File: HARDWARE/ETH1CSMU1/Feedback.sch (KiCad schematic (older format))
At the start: 91 parts, among them K301 CRR05-1A, K302 CRR05-1A, K303 CRR05-1A, K304 CRR05-1A, K305 CRR05-1A, K306 CRR05-1A, Q301 MMBT6429, Q302 MMBT6429, Q303 MMBT6429, Q304 MMBT6429, Q305 Q_NJFET_DGS, Q306 Q_NJFET_DGS, Q307 Q_NJFET_DGS, U301 AD746, U302 AQY221, U303 AQY221, U304 AQY221, U305 AQY221, U306 AQY221, U307 AQY221, U308 ADA4530-1, U309 AD746, U310 AD744, U311 AQY221, U312 AQY221, U313 AD744, U314 AQY221, U315 AD744, U316 REF102CU, U317 OPA277

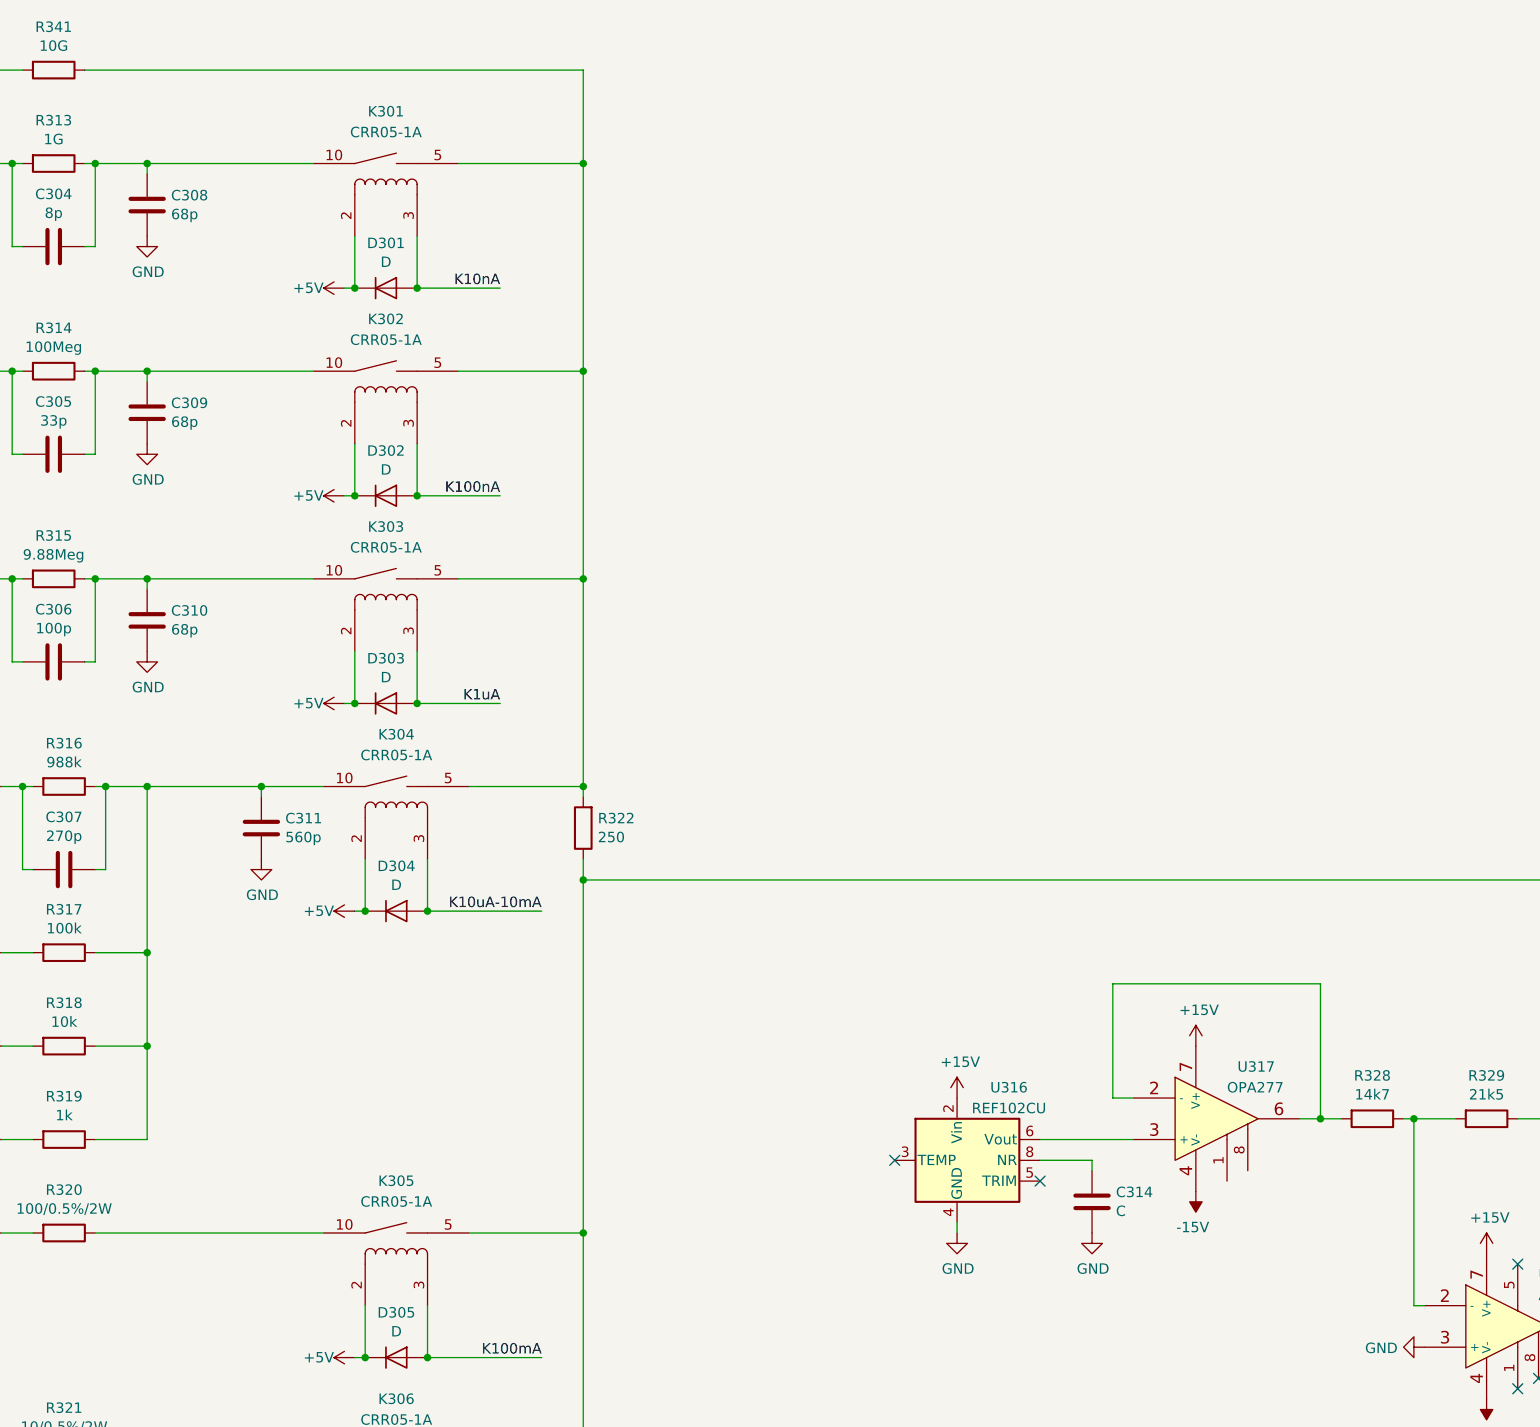
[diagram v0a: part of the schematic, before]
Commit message: Commit
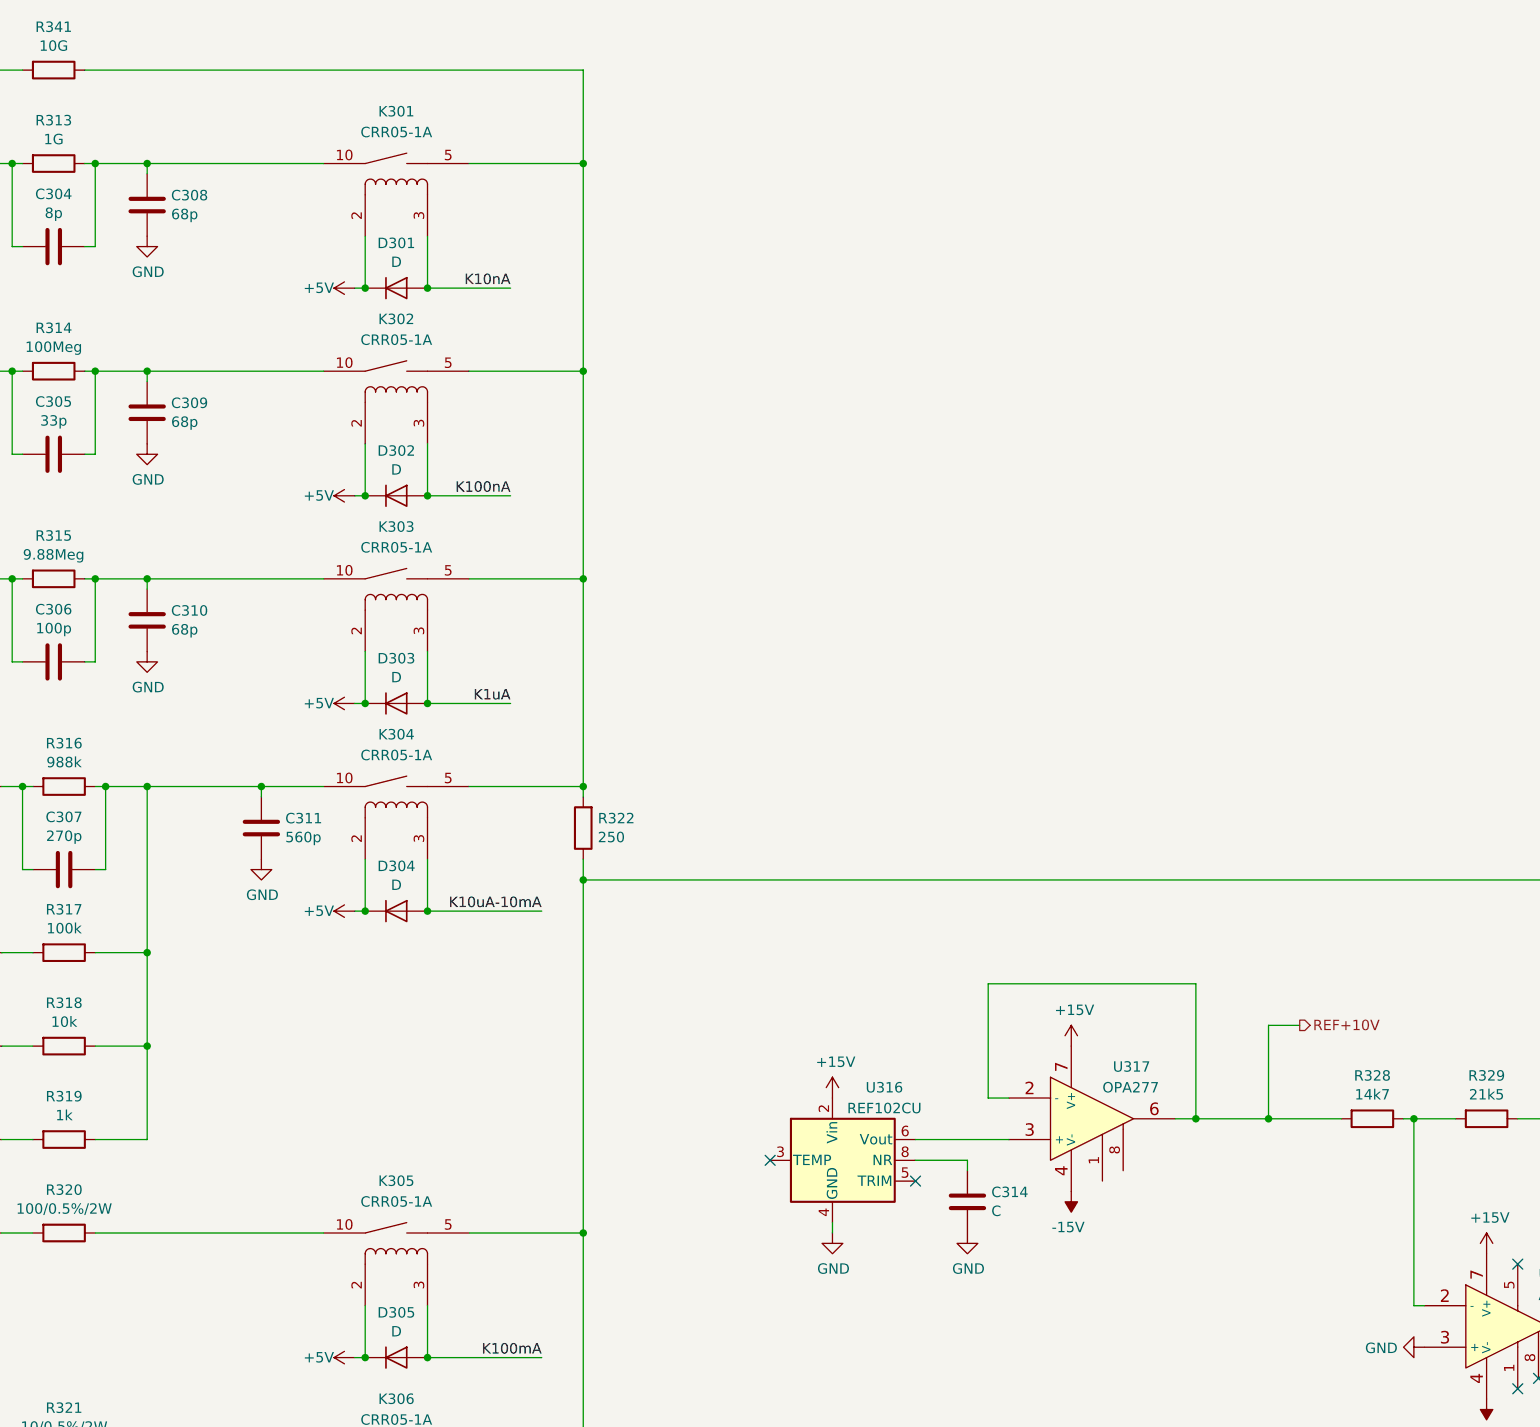
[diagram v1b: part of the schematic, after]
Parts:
- R310, R312, R318: footprint (none) -> SMD:R_0603_Symbol1
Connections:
- net REF+10V: now reaches R328.2, U317.2 (-), U317.6
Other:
- moved on the sheet: C314, D301, D302, D303, K301, K302, K303, U316, U317

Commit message: Footprints
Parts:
- C301, C302: footprint (none) -> SMD:C_0603_Symbol5
- C303, C304, C305, C308, C309, C310, C312: footprint (none) -> Capacitors_SMD:C_0603
- R305, R307, R309, R311, R317, R324: footprint (none) -> SMD:R_0603_Symbol3
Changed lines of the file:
@@
 F 0 "C305" V 5348 3300 50  0000 C CNN
 F 1 "33p" V 5439 3300 50  0000 C CNN
-F 2 "" H 5638 3150 50  0001 C CNN
+F 2 "Capacitors_SMD:C_0603" H 5638 3150 50  0001 C CNN
 F 3 "~" H 5600 3300 50  0001 C CNN
 	1    5600 3300
@@
 F 0 "R311" V 4143 8300 50  0000 C CNN
 F 1 "100k" V 4234 8300 50  0000 C CNN
-F 2 "" V 4280 8300 50  0001 C CNN
+F 2 "SMD:R_0603_Symbol3" V 4280 8300 50  0001 C CNN
 F 3 "~" H 4350 8300 50  0001 C CNN
 	1    4350 8300
@@
 F 0 "C302" V 4098 8650 50  0000 C CNN
 F 1 "15p" V 4189 8650 50  0000 C CNN
-F 2 "" H 4388 8500 50  0001 C CNN
+F 2 "SMD:C_0603_Symbol5" H 4388 8500 50  0001 C CNN
 F 3 "~" H 4350 8650 50  0001 C CNN
 	1    4350 8650
@@
 F 0 "R309" V 3743 8300 50  0000 C CNN
 F 1 "100k" V 3834 8300 50  0000 C CNN
-F 2 "" V 3880 8300 50  0001 C CNN
+F 2 "SMD:R_0603_Symbol3" V 3880 8300 50  0001 C CNN
 F 3 "~" H 3950 8300 50  0001 C CNN
 	1    3950 8300
@@
 F 0 "C301" V 3698 8650 50  0000 C CNN
 F 1 "15p" V 3789 8650 50  0000 C CNN
-F 2 "" H 3988 8500 50  0001 C CNN
+F 2 "SMD:C_0603_Symbol5" H 3988 8500 50  0001 C CNN
 F 3 "~" H 3950 8650 50  0001 C CNN
 	1    3950 8650
@@
 F 0 "C303" H 4665 9546 50  0000 L CNN
 F 1 "39p" H 4665 9455 50  0000 L CNN
-F 2 "" H 4588 9350 50  0001 C CNN
+F 2 "Capacitors_SMD:C_0603" H 4588 9350 50  0001 C CNN
 F 3 "~" H 4550 9500 50  0001 C CNN
 	1    4550 9500
@@
 F 0 "R307" V 2843 9100 50  0000 C CNN
 F 1 "100k" V 2934 9100 50  0000 C CNN
-F 2 "" V 2980 9100 50  0001 C CNN
+F 2 "SMD:R_0603_Symbol3" V 2980 9100 50  0001 C CNN
 F 3 "~" H 3050 9100 50  0001 C CNN
 	1    3050 9100
@@
 F 0 "R305" V 2193 8800 50  0000 C CNN
 F 1 "100k" V 2284 8800 50  0000 C CNN
-F 2 "" V 2330 8800 50  0001 C CNN
+F 2 "SMD:R_0603_Symbol3" V 2330 8800 50  0001 C CNN
 F 3 "~" H 2400 8800 50  0001 C CNN
 	1    2400 8800
@@
 F 0 "C309" H 6165 3146 50  0000 L CNN
 F 1 "68p" H 6165 3055 50  0000 L CNN
-F 2 "" H 6088 2950 50  0001 C CNN
+F 2 "Capacitors_SMD:C_0603" H 6088 2950 50  0001 C CNN
 F 3 "~" H 6050 3100 50  0001 C CNN
 	1    6050 3100
@@
 F 0 "C310" H 6165 4146 50  0000 L CNN
 F 1 "68p" H 6165 4055 50  0000 L CNN
-F 2 "" H 6088 3950 50  0001 C CNN
+F 2 "Capacitors_SMD:C_0603" H 6088 3950 50  0001 C CNN
 F 3 "~" H 6050 4100 50  0001 C CNN
 	1    6050 4100
@@
 F 0 "R317" V 5443 5700 50  0000 C CNN
 F 1 "100k" V 5534 5700 50  0000 C CNN
-F 2 "" V 5580 5700 50  0001 C CNN
+F 2 "SMD:R_0603_Symbol3" V 5580 5700 50  0001 C CNN
 F 3 "~" H 5650 5700 50  0001 C CNN
 	1    5650 5700
@@
 F 0 "C304" V 5348 2300 50  0000 C CNN
 F 1 "8p" V 5439 2300 50  0000 C CNN
-F 2 "" H 5638 2150 50  0001 C CNN
+F 2 "Capacitors_SMD:C_0603" H 5638 2150 50  0001 C CNN
 F 3 "~" H 5600 2300 50  0001 C CNN
 	1    5600 2300
@@
 F 0 "C308" H 6165 2146 50  0000 L CNN
 F 1 "68p" H 6165 2055 50  0000 L CNN
-F 2 "" H 6088 1950 50  0001 C CNN
+F 2 "Capacitors_SMD:C_0603" H 6088 1950 50  0001 C CNN
 F 3 "~" H 6050 2100 50  0001 C CNN
 	1    6050 2100
@@
 F 0 "R324" H 8220 8746 50  0000 L CNN
 F 1 "100k" H 8220 8655 50  0000 L CNN
-F 2 "" V 8080 8700 50  0001 C CNN
+F 2 "SMD:R_0603_Symbol3" V 8080 8700 50  0001 C CNN
 F 3 "~" H 8150 8700 50  0001 C CNN
 	1    8150 8700
@@
 F 0 "C312" H 8715 8746 50  0000 L CNN
 F 1 "33p" H 8715 8655 50  0000 L CNN
-F 2 "" H 8638 8550 50  0001 C CNN
+F 2 "Capacitors_SMD:C_0603" H 8638 8550 50  0001 C CNN
 F 3 "~" H 8600 8700 50  0001 C CNN
 	1    8600 8700
